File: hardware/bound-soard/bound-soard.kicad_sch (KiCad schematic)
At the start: 9 parts, among them J1 Signal_Input, J2 Conn_01x02_Female, J3 Conn_01x02_Male, J4 Conn_01x02_Female, J5 Supply, J6 Conn_01x02_Male, J7 Conn_01x02_Female, J8 Conn_01x02_Male, J9 Signal_Output

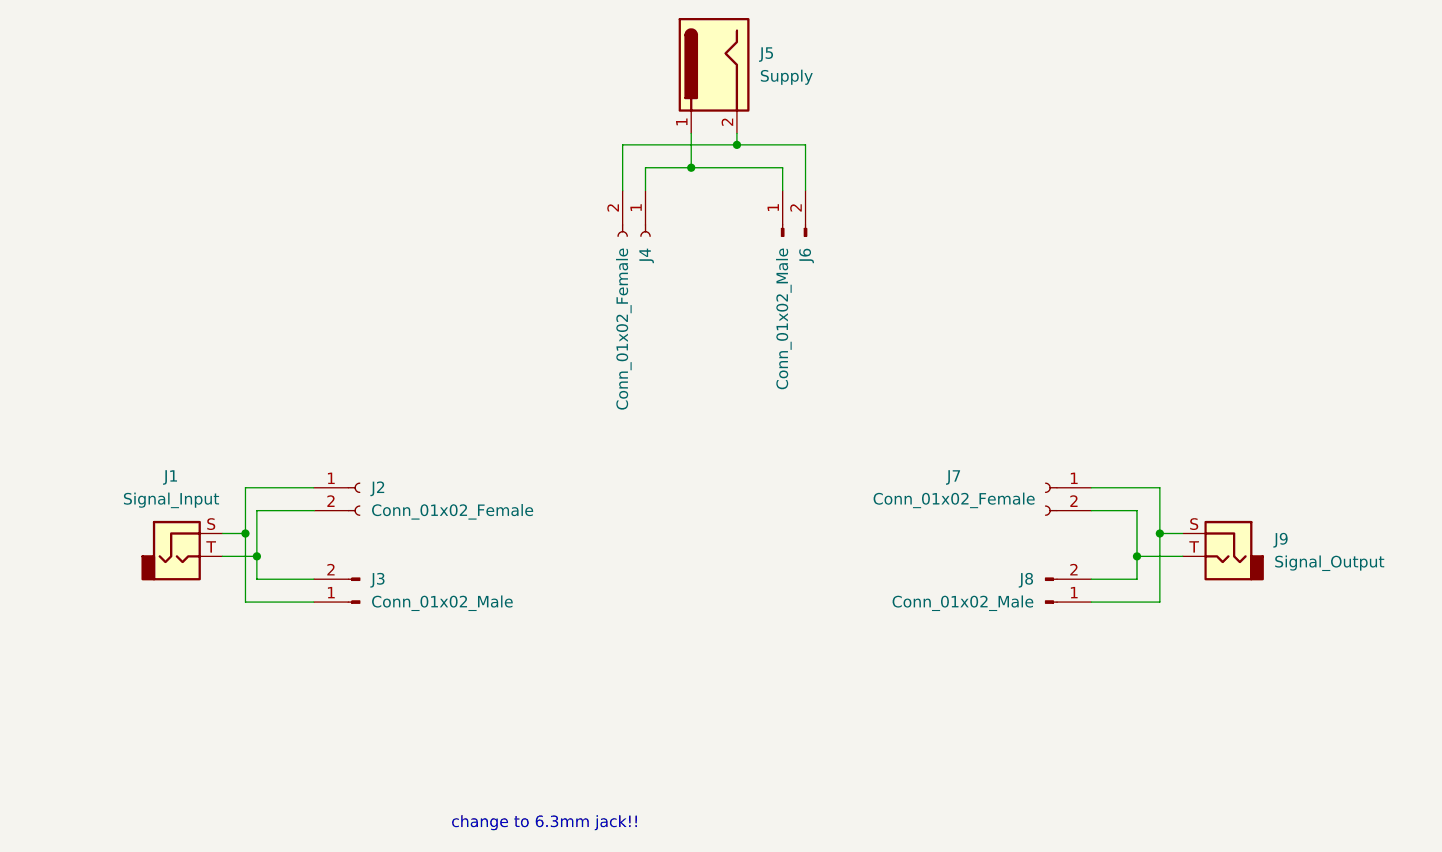
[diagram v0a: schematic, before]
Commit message: probably final
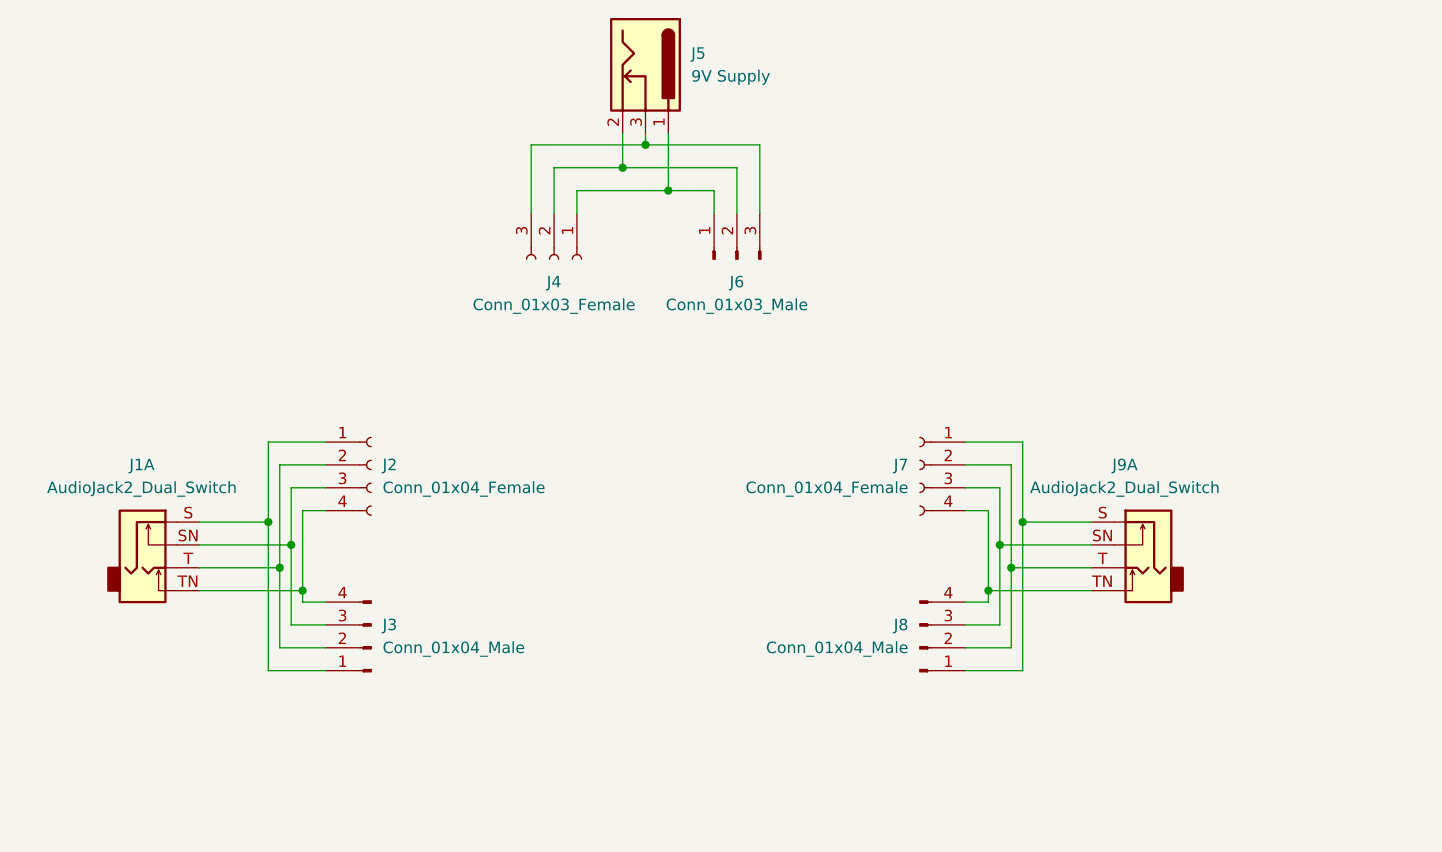
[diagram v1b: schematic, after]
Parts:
- removed J1: Signal_Input, Connector_Audio:Jack_6.35mm_Neutrik_NRJ4HF_Horizontal, symbol Connector:AudioJack2
- removed J2, J4, J7: Conn_01x02_Female, Connector_PinSocket_2.54mm:PinSocket_1x02_P2.54mm_Vertical, symbol Connector:Conn_01x02_Female
- removed J3, J6, J8: Conn_01x02_Male, Connector_PinHeader_2.54mm:PinHeader_1x02_P2.54mm_Vertical, symbol Connector:Conn_01x02_Male
- removed J5: Supply, Connector_BarrelJack:BarrelJack_Horizontal, symbol Connector:Jack-DC
- removed J9: Signal_Output, Connector_Audio:Jack_6.35mm_Neutrik_NRJ4HF_Horizontal, symbol Connector:AudioJack2
- added J1, J9: AudioJack2_Dual_Switch, Connector_Audio:Jack_6.35mm_Neutrik_NRJ4HF_Horizontal, symbol Connector:AudioJack2_Dual_Switch
- added J2, J7: Conn_01x04_Female, Connector_PinSocket_2.54mm:PinSocket_1x04_P2.54mm_Vertical, symbol Connector:Conn_01x04_Female
- added J3, J8: Conn_01x04_Male, Connector_PinHeader_2.54mm:PinHeader_1x04_P2.54mm_Vertical, symbol Connector:Conn_01x04_Male
- added J4: Conn_01x03_Female, Connector_PinSocket_2.54mm:PinSocket_1x03_P2.54mm_Vertical, symbol Connector:Conn_01x03_Female
- added J5: 9V Supply, Connector_BarrelJack:BarrelJack_Horizontal, symbol Connector:Barrel_Jack_Switch
- added J6: Conn_01x03_Male, Connector_PinHeader_2.54mm:PinHeader_1x03_P2.54mm_Vertical, symbol Connector:Conn_01x03_Male
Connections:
- new net: J1.S, J2.1 (Pin_1), J3.1 (Pin_1)
- new net: J1.SN, J2.3 (Pin_3), J3.3 (Pin_3)
- new net: J1.T, J2.2 (Pin_2), J3.2 (Pin_2)
- new net: J1.TN, J2.4 (Pin_4), J3.4 (Pin_4)
- new net: J4.1 (Pin_1), J5.1, J6.1 (Pin_1)
- new net: J4.2 (Pin_2), J5.2, J6.2 (Pin_2)
- new net: J4.3 (Pin_3), J5.3, J6.3 (Pin_3)
- new net: J7.1 (Pin_1), J8.1 (Pin_1), J9.S
- new net: J7.2 (Pin_2), J8.2 (Pin_2), J9.T
- new net: J7.3 (Pin_3), J8.3 (Pin_3), J9.SN
- new net: J7.4 (Pin_4), J8.4 (Pin_4), J9.TN
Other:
- note removed: "change to 6.3mm jack!!"
